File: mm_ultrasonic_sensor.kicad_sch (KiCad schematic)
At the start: 0 parts

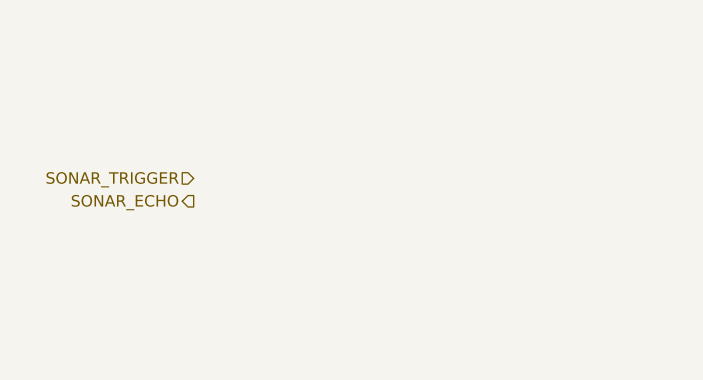
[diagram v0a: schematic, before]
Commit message: tp2
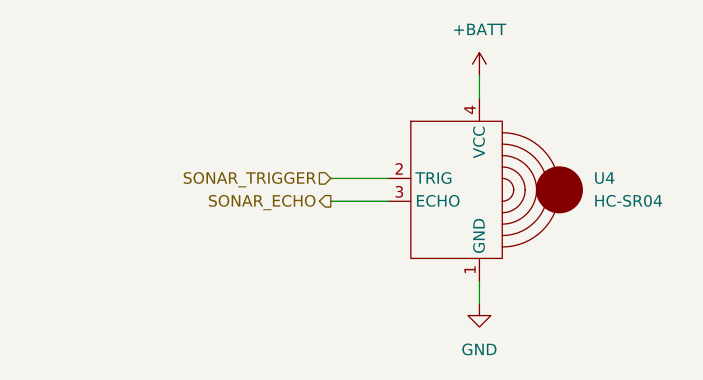
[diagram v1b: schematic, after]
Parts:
- added U4: HC-SR04, minimouse:HC-SR04, symbol minimouse:HC-SR04
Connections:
- net SONAR_ECHO: now also U4.3 (ECHO)
- net SONAR_TRIGGER: now also U4.2 (TRIG)
- new net +BATT: U4.4 (VCC)
- new net GND: U4.1 (GND)
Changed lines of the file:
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@@
 (kicad_sch (version 20230121) (generator eeschema)
   (paper "A4")
-  (hierarchical_label "SONAR_TRIGGER" (shape input) (at 109.22 88.9 180) (fields_autoplaced)
+  (wire (pts (xy 140.97 77.47) (xy 140.97 80.01))
+    (stroke (width 0) (type default))
+  )
+  (wire (pts (xy 124.46 88.9) (xy 130.81 88.9))
+    (stroke (width 0) (type default))
+  )
+  (wire (pts (xy 140.97 100.33) (xy 140.97 102.87))
+    (stroke (width 0) (type default))
+  )
+  (wire (pts (xy 124.46 91.44) (xy 130.81 91.44))
+    (stroke (width 0) (type default))
+  )
+  (hierarchical_label "SONAR_TRIGGER" (shape input) (at 124.46 88.9 180) (fields_autoplaced)
     (effects (font (size 1.27 1.27)) (justify right))
   )
-  (hierarchical_label "SONAR_ECHO" (shape output) (at 109.22 91.44 180) (fields_autoplaced)
+  (hierarchical_label "SONAR_ECHO" (shape output) (at 124.46 91.44 180) (fields_autoplaced)
     (effects (font (size 1.27 1.27)) (justify right))
   )
+  (symbol (lib_id "minimouse:HC-SR04") (at 140.97 90.17 0) (unit 1)
+    (in_bom yes) (on_board yes) (dnp no) (fields_autoplaced)
+    (property "Reference" "U4" (at 153.67 88.9 0)
+      (effects (font (size 1.27 1.27)) (justify left))
+    )
+    (property "Value" "HC-SR04" (at 153.67 91.44 0)
+      (effects (font (size 1.27 1.27)) (justify left))
+    )
+    (property "Footprint" "minimouse:HC-SR04" (at 140.97 90.17 0)
+      (effects (font (size 1.27 1.27)) hide)
+    )
+    (property "Datasheet" "" (at 140.97 90.17 0)
+      (effects (font (size 1.27 1.27)) hide)
+    )
+    (pin "1")
+    (pin "2")
+    (pin "3")
+    (pin "4")
+    (instances
+      (project "minimouse"
+        (path "/d8fa4cba-2469-4231-847f-065b6b829f44/224298a9-7d6e-4a70-a0a5-f2614895ec28"
+          (reference "U4") (unit 1)
+        )
+      )
+    )
+  )
+  (symbol (lib_id "power:+BATT") (at 140.97 77.47 0) (unit 1)
+    (in_bom yes) (on_board yes) (dnp no) (fields_autoplaced)
+    (property "Reference" "#PWR024" (at 140.97 81.28 0)
+      (effects (font (size 1.27 1.27)) hide)
+    )
+    (property "Value" "+BATT" (at 140.97 72.39 0)
+      (effects (font (size 1.27 1.27)))
+    )
+    (property "Footprint" "" (at 140.97 77.47 0)
+      (effects (font (size 1.27 1.27)) hide)
+    )
+    (property "Datasheet" "" (at 140.97 77.47 0)
+      (effects (font (size 1.27 1.27)) hide)
+    )
+    (pin "1")
+    (instances
+      (project "minimouse"
+        (path "/d8fa4cba-2469-4231-847f-065b6b829f44/224298a9-7d6e-4a70-a0a5-f2614895ec28"
+          (reference "#PWR024") (unit 1)
+        )
+      )
+    )
+  )
+  (symbol (lib_id "power:GND") (at 140.97 102.87 0) (unit 1)
+    (in_bom yes) (on_board yes) (dnp no) (fields_autoplaced)
+    (property "Reference" "#PWR025" (at 140.97 109.22 0)
+      (effects (font (size 1.27 1.27)) hide)
+    )
+    (property "Value" "GND" (at 140.97 107.95 0)
+      (effects (font (size 1.27 1.27)))
+    )
+    (property "Footprint" "" (at 140.97 102.87 0)
+      (effects (font (size 1.27 1.27)) hide)
+    )
+    (property "Datasheet" "" (at 140.97 102.87 0)
+      (effects (font (size 1.27 1.27)) hide)
+    )
+    (pin "1")
+    (instances
+      (project "minimouse"
+        (path "/d8fa4cba-2469-4231-847f-065b6b829f44/224298a9-7d6e-4a70-a0a5-f2614895ec28"
+          (reference "#PWR025") (unit 1)
+        )
+      )
+    )
+  )
 )
